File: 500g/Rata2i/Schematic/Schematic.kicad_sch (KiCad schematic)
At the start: 7 parts, among them J1 Screw_Terminal_01x03, J2 Screw_Terminal_01x03, J3 Screw_Terminal_01x03, J4 Screw_Terminal_01x03, J5 Screw_Terminal_01x03, J7 Screw_Terminal_01x03, U1 DEV-16771

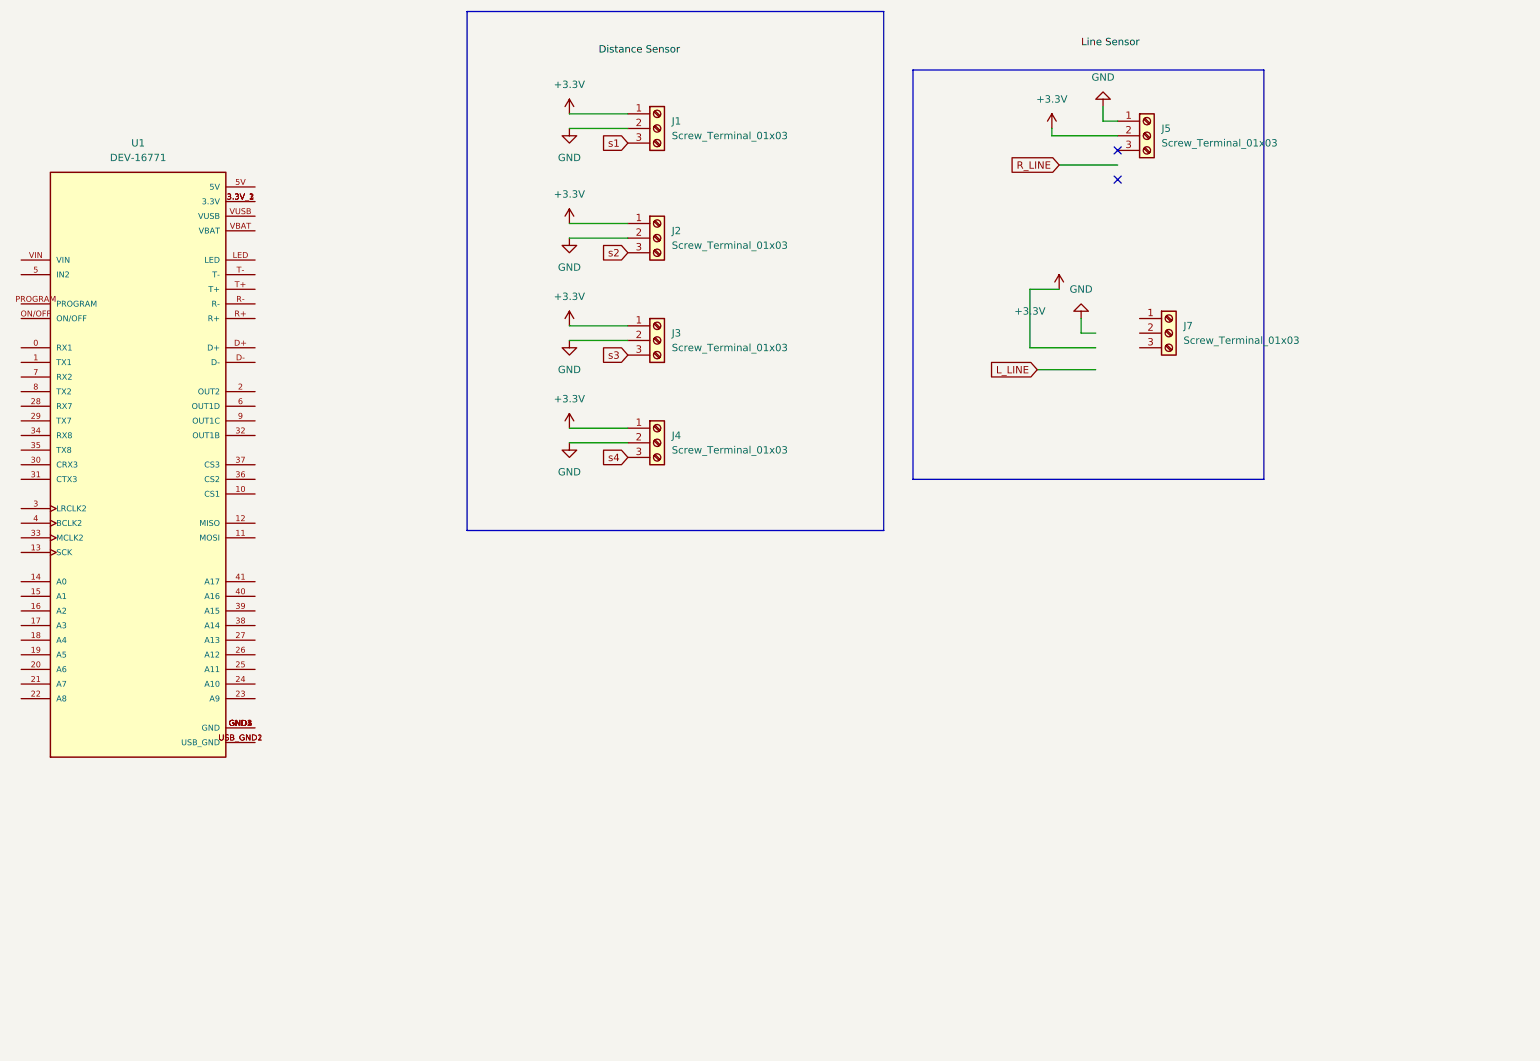
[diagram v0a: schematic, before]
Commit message: Updated Rata2i schematic
Now with more stuff! And 1 (one) LED
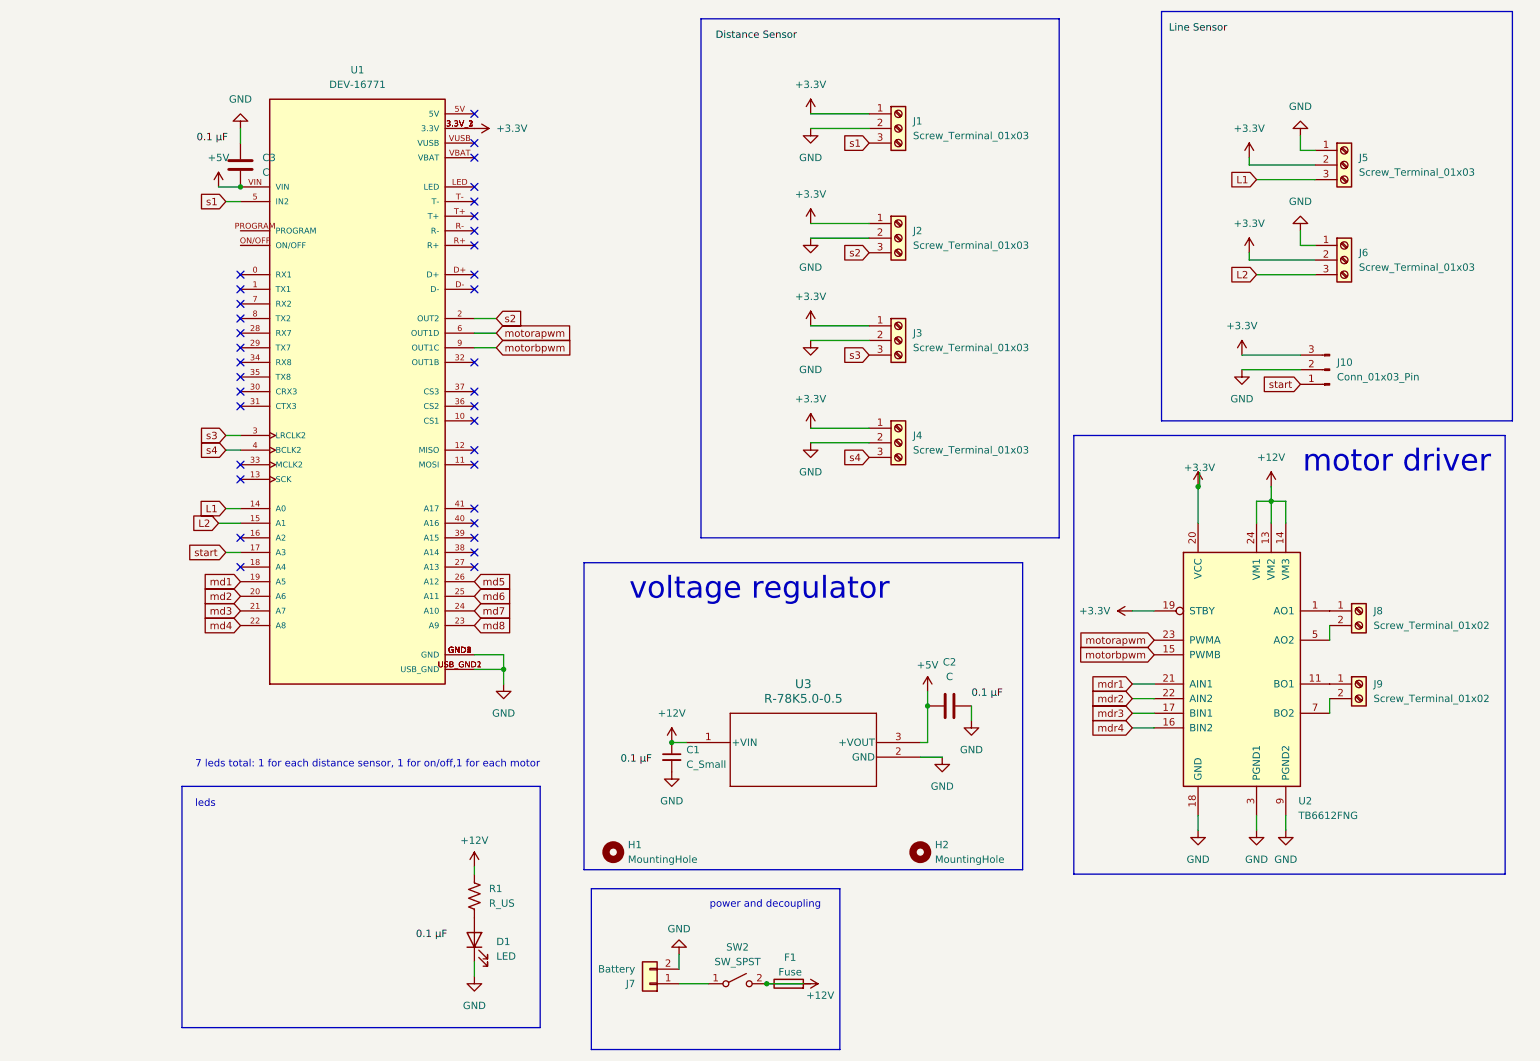
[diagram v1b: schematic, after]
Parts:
- added C1: C_Small, symbol Device:C_Small
- added C2, C3: C, symbol Device:C
- added D1: LED, symbol Device:LED
- added F1: Fuse, symbol Device:Fuse
- added H1, H2: MountingHole, symbol Mechanical:MountingHole
- added J10: Conn_01x03_Pin, symbol Connector:Conn_01x03_Pin
- added J7: Battery, symbol Connector_Generic:Conn_01x02
- added J8, J9: Screw_Terminal_01x02, symbol Connector:Screw_Terminal_01x02
- added R1: R_US, symbol Device:R_US
- added SW2: SW_SPST, symbol Switch:SW_SPST
- added U2: TB6612FNG, Package_SO:SSOP-24_5.3x8.2mm_P0.65mm, symbol Driver_Motor:TB6612FNG
- added U3: R-78K5.0-0.5, SIP3_R-78K-0.5_RCP, symbol 2024-11-08_01-03-56:R-78K5.0-0.5
- renumbered J7 to J6
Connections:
- net +3.3V: now also J6.2 (Pin_2), U1.3.3V_1 (3.3V), U1.3.3V_2 (3.3V), U1.3.3V_3 (3.3V), J10.3 (Pin_3), U2.19 (STBY), U2.20 (VCC)
- net GND: now also J6.1 (Pin_1), U1.GND1 (GND), U1.GND2 (GND), U1.GND3 (GND), U1.GND4 (GND), U1.GND5 (GND), U1.USB_GND1 (USB_GND), U1.USB_GND2 (USB_GND), C1.2, C2.2, C3.1, D1.1 (K), J10.2 (Pin_2), J7.2 (Pin_2), U2.10 (PGND2), U2.18 (GND), U2.3 (PGND1), U2.4 (PGND1), U2.9 (PGND2), U3.2 (GND)
- net s1: now also U1.5 (IN2)
- net s2: now also U1.2 (OUT2)
- net s3: now also U1.3 (LRCLK2)
- net s4: now also U1.4 (BCLK2)
- net L2: now reaches J6.3 (Pin_3)
- net L2: now also U1.15 (A1)
- net L1: now reaches U1.14 (A0)
- net L1: now also J5.3 (Pin_3)
- net start: now reaches U1.17 (A3)
- net start: now also J10.1 (Pin_1)
- net md1: now reaches U1.19 (A5)
- net md2: now reaches U1.20 (A6)
- net md3: now reaches U1.21 (A7)
- net md4: now reaches U1.22 (A8)
- net md8: now reaches U1.23 (A9)
- net md7: now reaches U1.24 (A10)
- net md6: now reaches U1.25 (A11)
- net md5: now reaches U1.26 (A12)
- net motorapwm: now reaches U1.6 (OUT1D)
- net motorapwm: now also U2.23 (PWMA)
- net motorbpwm: now reaches U1.9 (OUT1C)
- net motorbpwm: now also U2.15 (PWMB)
- net +5V: now reaches U1.VIN
- net +5V: now also C2.1, C3.2, U3.3 (+VOUT)
- new net: D1.2 (A), R1.2
- new net: J9.1 (Pin_1), U2.11 (BO1), U2.12 (BO1)
- new net: J9.2 (Pin_2), U2.7 (BO2), U2.8 (BO2)
- new net: J8.1 (Pin_1), U2.1 (AO1), U2.2 (AO1)
- new net: J8.2 (Pin_2), U2.5 (AO2), U2.6 (AO2)
- new net: J7.1 (Pin_1), SW2.1 (A)
- new net +12V: C1.1, F1.1, R1.1, SW2.2 (B), U2.13 (VM2), U2.14 (VM3), U2.24 (VM1), U3.1 (+VIN)
- new net mdr1: U2.21 (AIN1)
- new net mdr2: U2.22 (AIN2)
- new net mdr3: U2.17 (BIN1)
- new net mdr4: U2.16 (BIN2)
- no-connect marks 2 -> 35
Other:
- note added: "7 leds total: 1 for each distance sensor, 1 for on/off,1 for each motor"
- note added: "leds"
- note added: "motor driver"
- note added: "power and decoupling"
- note added: "voltage regulator"
- moved on the sheet: J1, J2, J3, J4, J6, U1
